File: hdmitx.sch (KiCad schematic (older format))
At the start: 52 parts, among them J4 HDMI_CONN, U15 TLV70018, U16 TLV70018, U3 IT6613, U8 PCM1862, Y2 24.576MHz

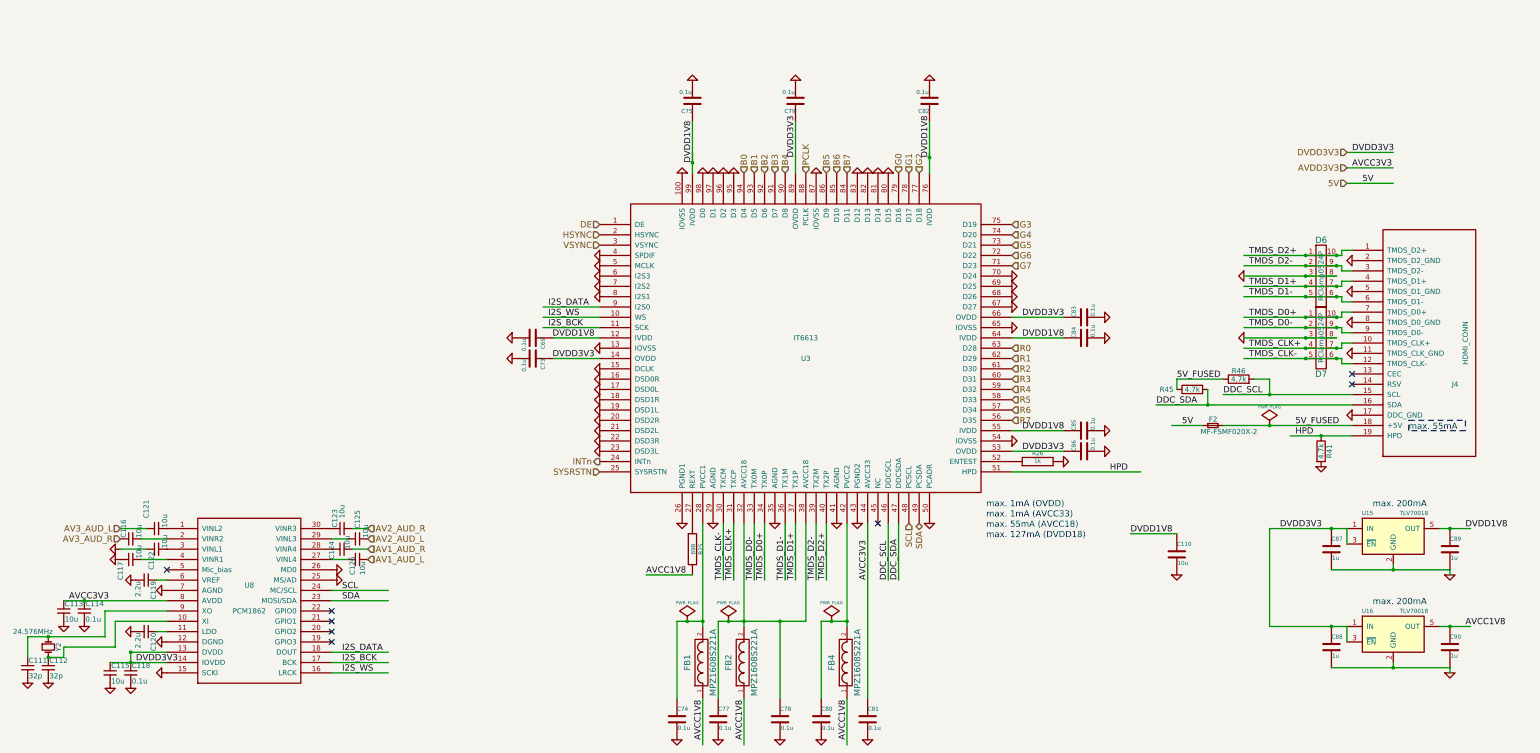
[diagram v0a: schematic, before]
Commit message: finalize pcb v1.6
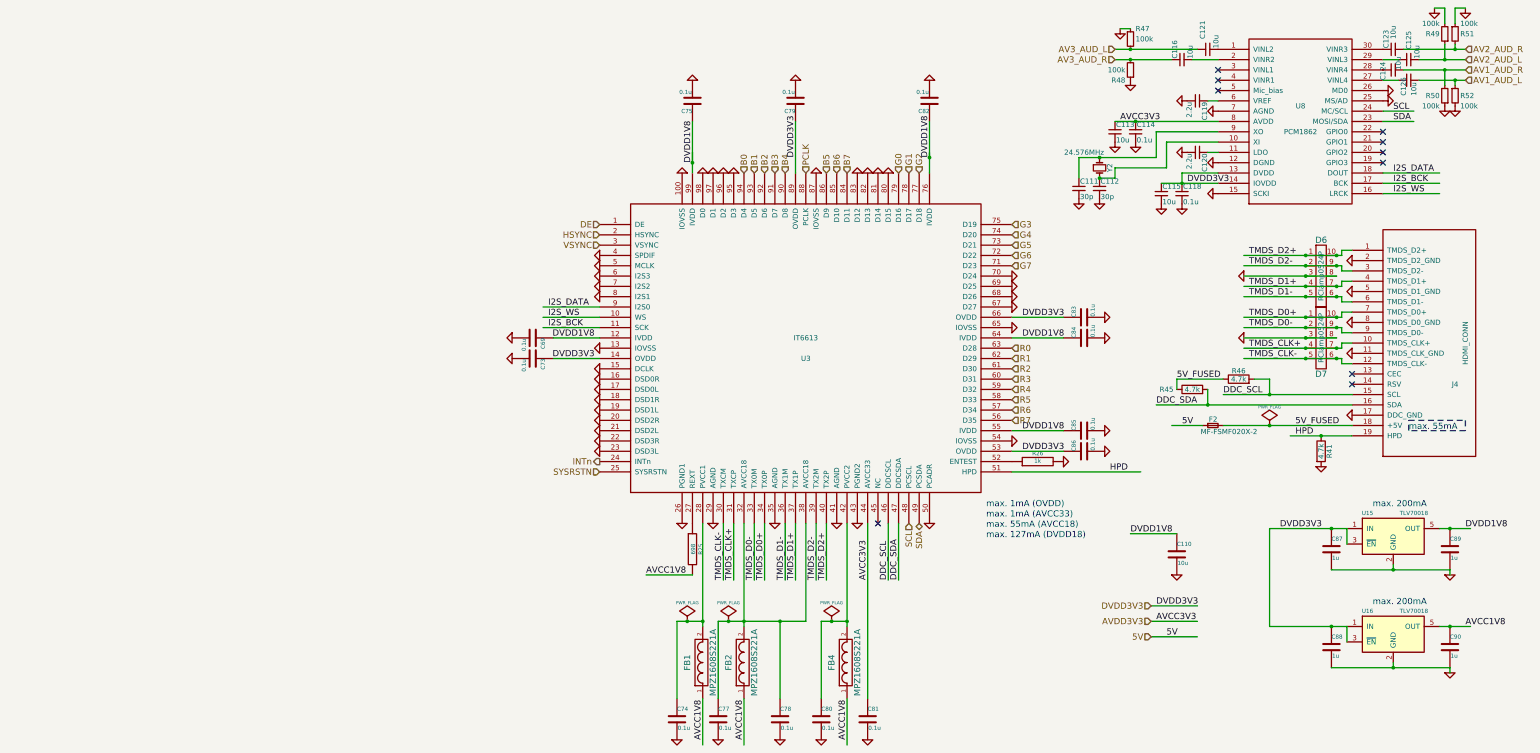
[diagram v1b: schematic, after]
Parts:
- removed C117, C122: 10u, custom_components:SM0603_Capa_libcms, symbol C_Small
- added R47, R48, R49, R50, R51, R52: 100k, custom_components:SM0603_Resistor_libcms, symbol R_Small
- C111, C112: value 32p -> 30p
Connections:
- wire segments 122 -> 132
- no-connect marks 8 -> 10
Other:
- moved on the sheet: C111, C112, C113, C114, C115, C116, C118, C119, C120, C121, C123, C124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

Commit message: - Update schematics and board to KiCAD 5.x
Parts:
- C110, C69, C73, C74, C75, C77, C78, C79, C80, C81, C82, C83, C84, C85, C86, C87, C88, C89, C90: symbol C-RESCUE-ossc_board -> ossc_board-rescue:C-RESCUE-ossc_board
- C111, C112, C113, C114, C115, C116, C118, C119, C120, C121, C123, C124, C125, C126: symbol C_Small -> ossc_board-rescue:C_Small
- D6, D7: symbol RClamp0524P -> ossc_board-rescue:RClamp0524P
- F2: symbol F_Small -> ossc_board-rescue:F_Small
- FB1, FB2, FB4: symbol FILTER -> ossc_board-rescue:FILTER
- J4: symbol HDMI_CONN -> ossc_board-rescue:HDMI_CONN
- R25, R26: symbol R-RESCUE-ossc_board -> ossc_board-rescue:R-RESCUE-ossc_board
- R41, R45, R46: symbol R -> ossc_board-rescue:R
- R47, R48, R49, R50, R51, R52: symbol R_Small -> ossc_board-rescue:R_Small
- U15, U16: symbol TLV71209DBV-RESCUE-ossc_board -> ossc_board-rescue:TLV71209DBV-RESCUE-ossc_board
- U3: symbol IT6613 -> ossc_board-rescue:IT6613
- U8: symbol PCM1862 -> ossc_board-rescue:PCM1862
- Y2: symbol Crystal_Small -> ossc_board-rescue:Crystal_Small
